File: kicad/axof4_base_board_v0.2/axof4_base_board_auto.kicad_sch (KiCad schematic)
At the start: 1 part

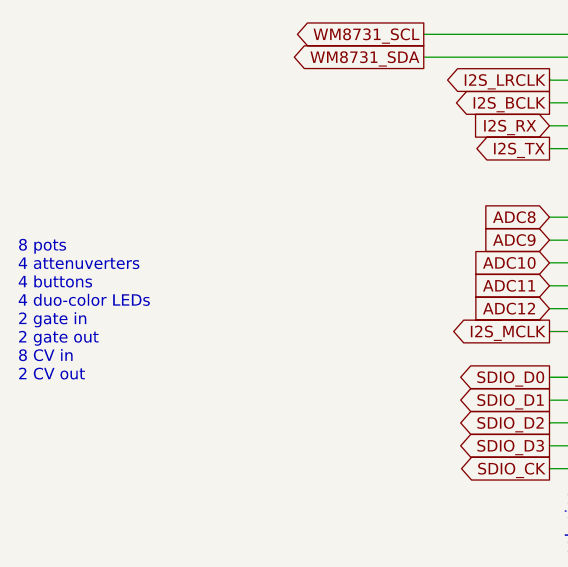
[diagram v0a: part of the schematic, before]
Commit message: working towards own F427 daughterboard
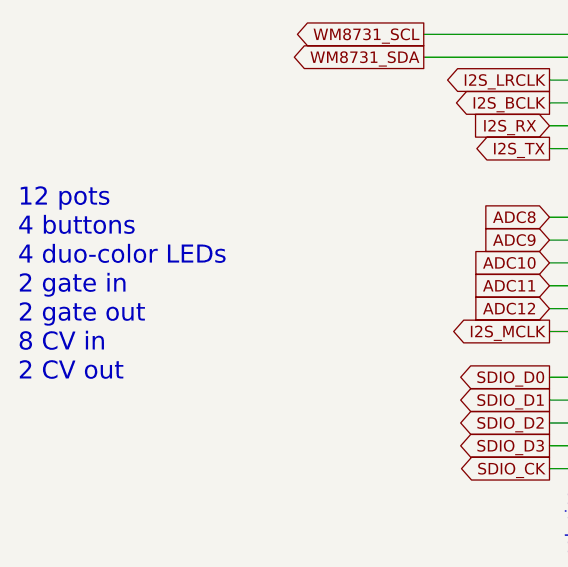
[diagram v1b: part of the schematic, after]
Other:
- note added: "12 pots 4 buttons 4 duo-color LEDs 2 gate in 2 gate out 8 CV in 2 CV out"
- note removed: "8 pots 4 attenuverters 4 buttons 4 duo-color LEDs 2 gate in 2 gate out 8 CV in 2 CV out"
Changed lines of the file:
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@@
     (effects (font (size 1.27 1.27)) (justify left bottom))
   )
-  (text "8 pots\n4 attenuverters\n4 buttons\n4 duo-color LEDs\n2 gate in\n2 gate out\n8 CV in\n2 CV out"
+  (text "12 pots\n4 buttons\n4 duo-color LEDs\n2 gate in\n2 gate out\n8 CV in\n2 CV out"
     (at 56.515 151.765 0)
-    (effects (font (size 1.27 1.27)) (justify left bottom))
+    (effects (font (size 2 2)) (justify left bottom))
   )
   (text "done" (at 266.065 132.715 0)
@@
       (reference "#PWR0164") (unit 1) (value "+12V") (footprint "")
     )
+    (path "/00000000-0000-0000-0000-00005ed86ed4/f81894ec-f168-4612-bfcd-ec16efa1d002"
+      (reference "#PWR0165") (unit 1) (value "+12V") (footprint "")
+    )
     (path "/00000000-0000-0000-0000-00005ed86ed4/14cc8e54-6739-4c6f-a4bf-829f53e763f8"
-      (reference "#PWR?") (unit 1) (value "GND") (footprint "")
-    )
-    (path "/00000000-0000-0000-0000-00005ed86ed4/f81894ec-f168-4612-bfcd-ec16efa1d002"
-      (reference "#PWR?") (unit 1) (value "+12V") (footprint "")
+      (reference "#PWR0166") (unit 1) (value "GND") (footprint "")
     )
     (path "/00000000-0000-0000-0000-00005efc127a/00000000-0000-0000-0000-0000627664b7"
@@
     )
     (path "/00000000-0000-0000-0000-00005ed86ed4/48ff0ceb-ea44-48a3-b980-0dcbba8daca9"
-      (reference "C?") (unit 1) (value "10uF") (footprint "Capacitor_SMD:C_1206_3216Metric")
+      (reference "C63") (unit 1) (value "10uF") (footprint "Capacitor_SMD:C_1206_3216Metric")
     )
     (path "/00000000-0000-0000-0000-00005ed86ed4/eb4bcba5-eacd-4d10-b48f-42efb5537651"
-      (reference "C?") (unit 1) (value "100nF") (footprint "Capacitor_SMD:C_0603_1608Metric_Pad1.08x0.95mm_HandSolder")
+      (reference "C64") (unit 1) (value "100nF") (footprint "Capacitor_SMD:C_0603_1608Metric_Pad1.08x0.95mm_HandSolder")
     )
     (path "/00000000-0000-0000-0000-00005ed86ed4/00000000-0000-0000-0000-000061cfe23a"
@@
     )
     (path "/00000000-0000-0000-0000-00005ed86ed4/87ff1ff0-74ca-46c8-a8d5-9c57b605095f"
-      (reference "FB?") (unit 1) (value "100 ohm @ 100 Mhz") (footprint "Resistor_SMD:R_0805_2012Metric")
+      (reference "FB4") (unit 1) (value "100 ohm @ 100 Mhz") (footprint "Resistor_SMD:R_0805_2012Metric")
     )
     (path "/00000000-0000-0000-0000-00005ecd8b86/00000000-0000-0000-0000-000062811874"
-      (reference "J1") (unit 1) (value "Micro_SD_Card") (footprint "foots:PJS008U-3000-0")
+      (reference "J1") (unit 1) (value "Micro_SD_Card") (footprint "foots:Sofng_TF-15x15_sd_card_socket")
     )
     (path "/00000000-0000-0000-0000-00005ed86ed4/00000000-0000-0000-0000-000061cbfa5a"
@@
     )
     (path "/00000000-0000-0000-0000-00005efc127a/00000000-0000-0000-0000-000061619d0f"
-      (reference "R5") (unit 1) (value "220") (footprint "Resistor_SMD:R_0603_1608Metric_Pad0.98x0.95mm_HandSolder")
+      (reference "R5") (unit 1) (value "33") (footprint "Resistor_SMD:R_0603_1608Metric_Pad0.98x0.95mm_HandSolder")
     )
     (path "/00000000-0000-0000-0000-00005efc127a/00000000-0000-0000-0000-00005efd0743"
@@
     )
     (path "/00000000-0000-0000-0000-00005ed86ed4/65e8bb0a-f088-4d66-b5bd-3e492b575a78"
-      (reference "U?") (unit 1) (value "LM1117-3.3") (footprint "foots:SOT-89-3_clearance")
+      (reference "U17") (unit 1) (value "LM1117-3.3") (footprint "foots:SOT-89-3_clearance")
     )
     (path "/00000000-0000-0000-0000-00005efc127a/00000000-0000-0000-0000-00005efd07f3"
